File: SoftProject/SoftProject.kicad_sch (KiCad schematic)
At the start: 37 parts, among them J1 USB_B_Micro, Q1 2N2219, Q2 2N2219, SW1 SW_Push, SW2 SW_Push, U1 ESP32-S2-WROVER, U2 AMS1117, U3 CP2102N-Axx-xQFN28

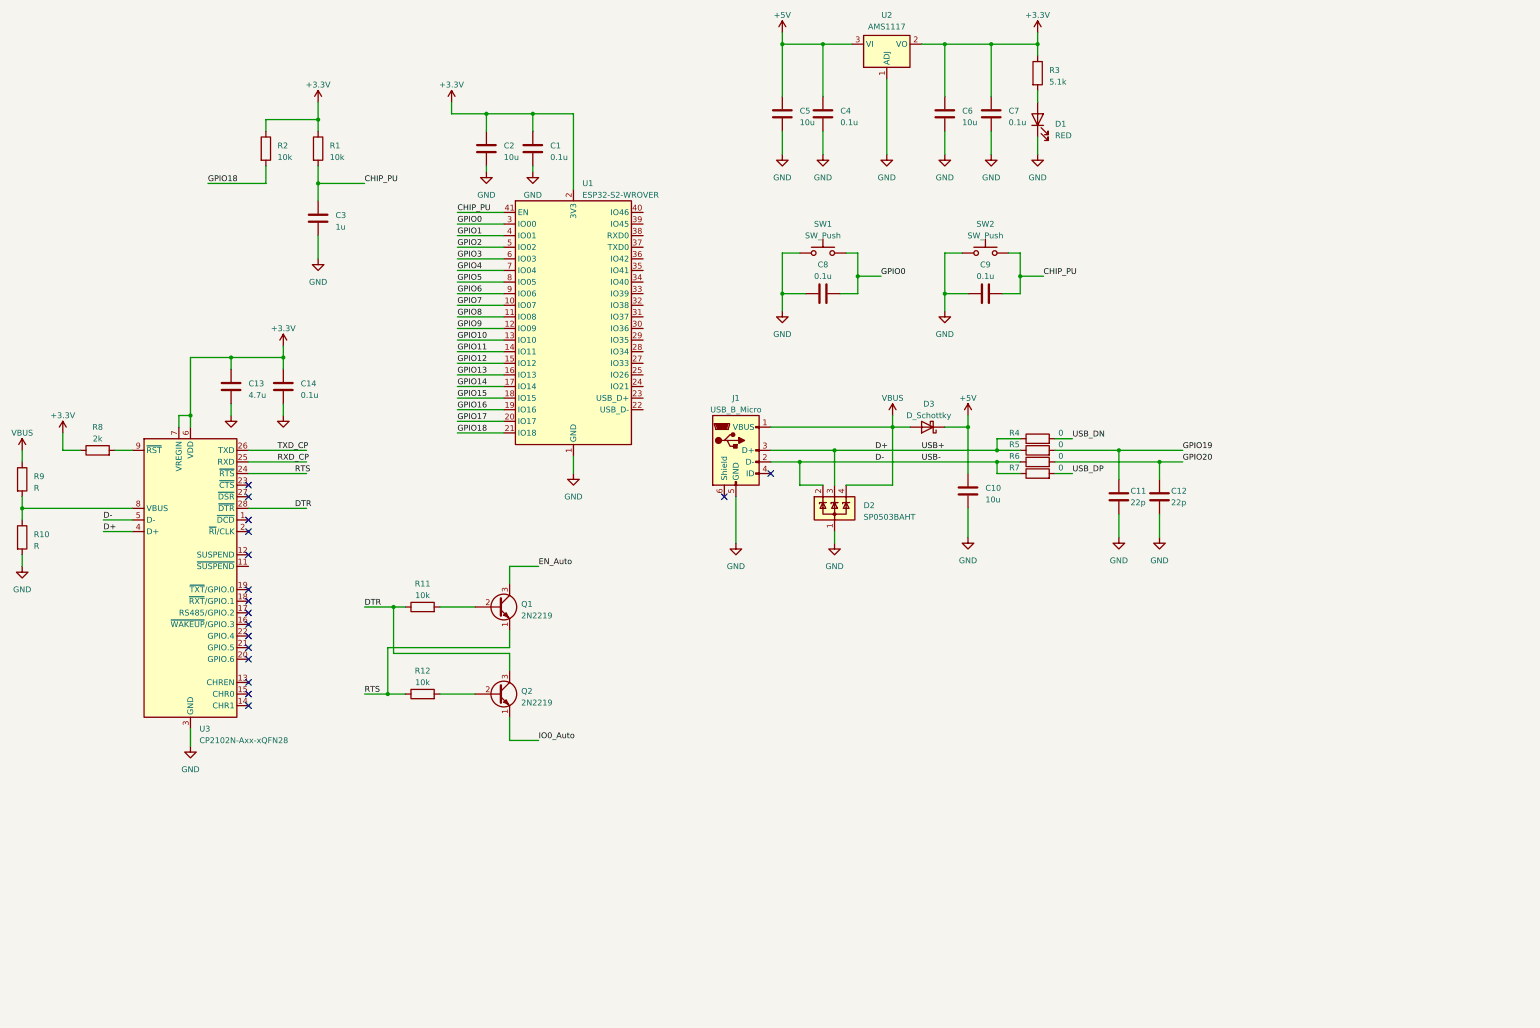
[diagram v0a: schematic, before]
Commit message: Finished schematic
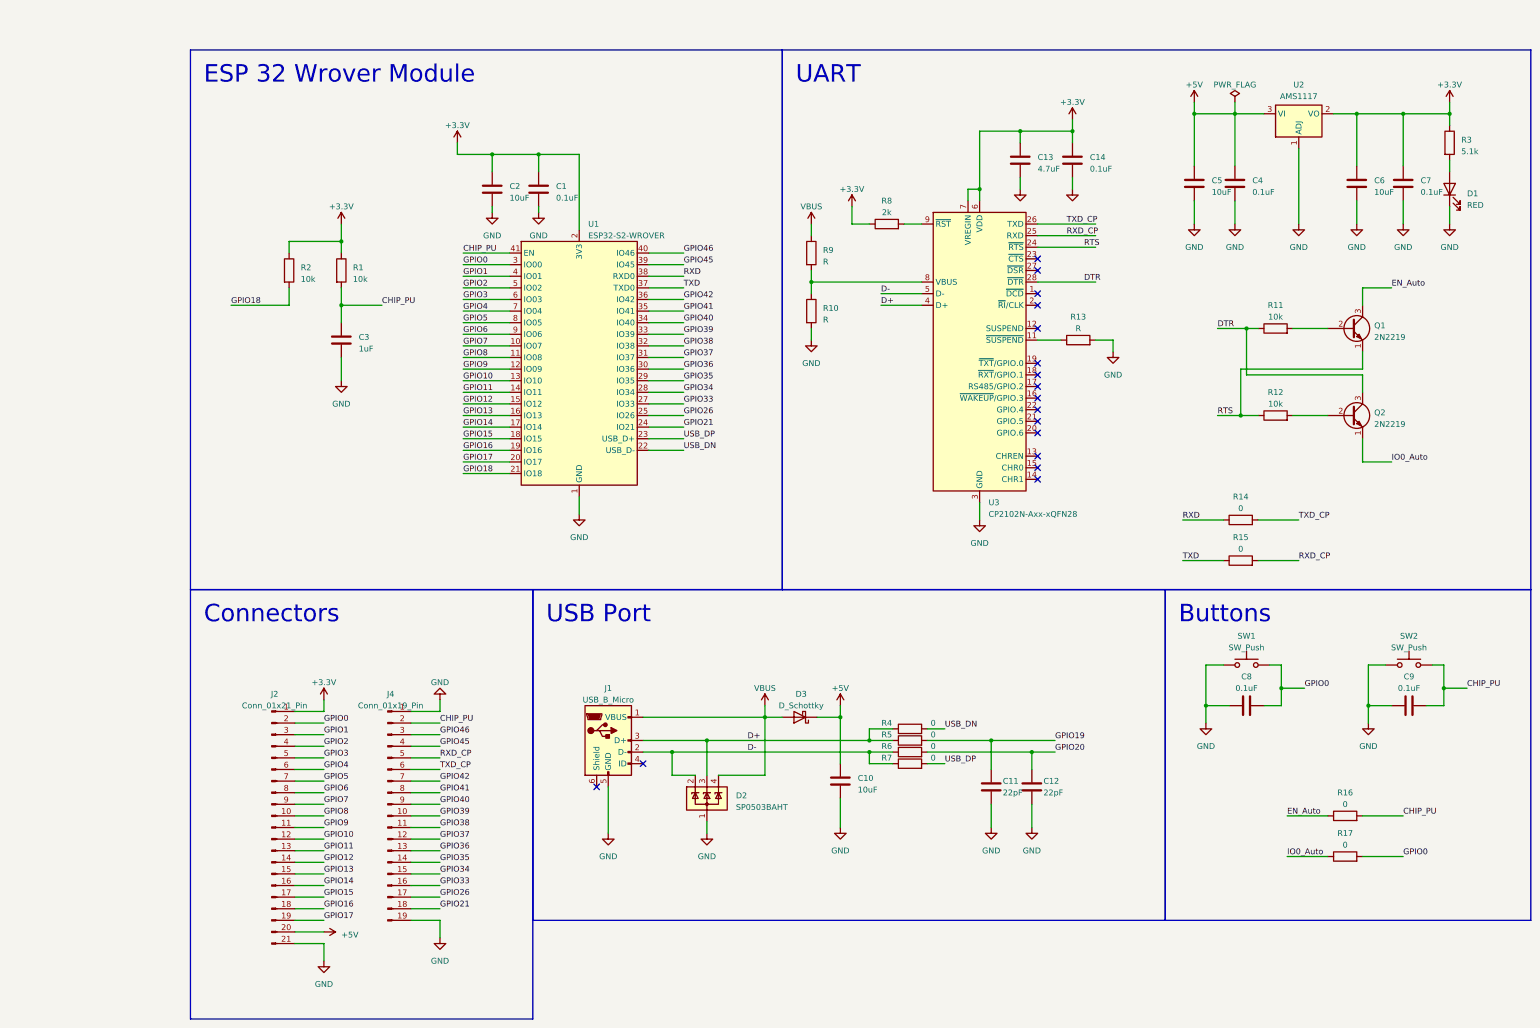
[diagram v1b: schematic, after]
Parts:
- added J2: Conn_01x21_Pin, symbol Connector:Conn_01x21_Pin
- added J4: Conn_01x19_Pin, symbol Connector:Conn_01x19_Pin
- added R13: R, symbol Device:R
- added R14, R15, R16, R17: 0, symbol Device:R
- C1, C14, C4, C7, C8, C9: value 0.1u -> 0.1uF
- C10, C2, C5, C6: value 10u -> 10uF
- C11, C12: value 22p -> 22pF
- C13: value 4.7u -> 4.7uF
- C3: value 1u -> 1uF
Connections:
- net +3.3V: now also J2.1 (Pin_1)
- net +5V: now also J2.20 (Pin_20)
- net CHIP_PU: now also J4.2 (Pin_2), R16.2
- net EN_Auto: now also R16.1
- net GND: now also J2.21 (Pin_21), J4.1 (Pin_1), J4.19 (Pin_19), R13.2
- net GPIO0: now also J2.2 (Pin_2), R17.2
- net GPIO1: now also J2.3 (Pin_3)
- net GPIO10: now also J2.12 (Pin_12)
- net GPIO11: now also J2.13 (Pin_13)
- net GPIO12: now also J2.14 (Pin_14)
- net GPIO13: now also J2.15 (Pin_15)
- net GPIO14: now also J2.16 (Pin_16)
- net GPIO15: now also J2.17 (Pin_17)
- net GPIO16: now also J2.18 (Pin_18)
- net GPIO17: now also J2.19 (Pin_19)
- net GPIO2: now also J2.4 (Pin_4)
- net GPIO3: now also J2.5 (Pin_5)
- net GPIO4: now also J2.6 (Pin_6)
- net GPIO5: now also J2.7 (Pin_7)
- net GPIO6: now also J2.8 (Pin_8)
- net GPIO7: now also J2.9 (Pin_9)
- net GPIO8: now also J2.10 (Pin_10)
- net GPIO9: now also J2.11 (Pin_11)
- net IO0_Auto: now also R17.1
- net RXD_CP: now also J4.5 (Pin_5), R15.2
- net TXD_CP: now also J4.6 (Pin_6), R14.2
- net USB_DN: now also U1.22 (USB_D-)
- net USB_DP: now also U1.23 (USB_D+)
- net at U3.11 (~{SUSPEND}): now also R13.1
- net GPIO21: now reaches U1.24 (IO21)
- net GPIO21: now also J4.18 (Pin_18)
- net GPIO26: now reaches U1.25 (IO26)
- net GPIO26: now also J4.17 (Pin_17)
- net GPIO33: now reaches U1.27 (IO33)
- net GPIO33: now also J4.16 (Pin_16)
- net GPIO34: now reaches U1.28 (IO34)
- net GPIO34: now also J4.15 (Pin_15)
- net GPIO35: now reaches U1.29 (IO35)
- net GPIO35: now also J4.14 (Pin_14)
- net GPIO36: now reaches U1.30 (IO36)
- net GPIO36: now also J4.13 (Pin_13)
- net GPIO37: now reaches U1.31 (IO37)
- net GPIO37: now also J4.12 (Pin_12)
- net GPIO38: now reaches U1.32 (IO38)
- net GPIO38: now also J4.11 (Pin_11)
- net GPIO39: now reaches U1.33 (IO39)
- net GPIO39: now also J4.10 (Pin_10)
- net GPIO40: now reaches U1.34 (IO40)
- net GPIO40: now also J4.9 (Pin_9)
- net GPIO41: now reaches U1.35 (IO41)
- net GPIO41: now also J4.8 (Pin_8)
- net GPIO42: now reaches U1.36 (IO42)
- net GPIO42: now also J4.7 (Pin_7)
- net TXD: now reaches U1.37 (TXD0)
- net TXD: now also R15.1
- net RXD: now reaches U1.38 (RXD0)
- net RXD: now also R14.1
- net GPIO45: now reaches U1.39 (IO45)
- net GPIO45: now also J4.4 (Pin_4)
- net GPIO46: now reaches U1.40 (IO46)
- net GPIO46: now also J4.3 (Pin_3)
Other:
- moved on the sheet: C1, C10, C11, C12, C13, C14, C2, C3, C4, C5, C6, C7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
